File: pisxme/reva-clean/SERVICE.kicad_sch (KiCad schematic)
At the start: 5 parts, among them J4 10171746-00021LF, U8 USB2 connector-boundary ESD, X8 SERVICE_Contract

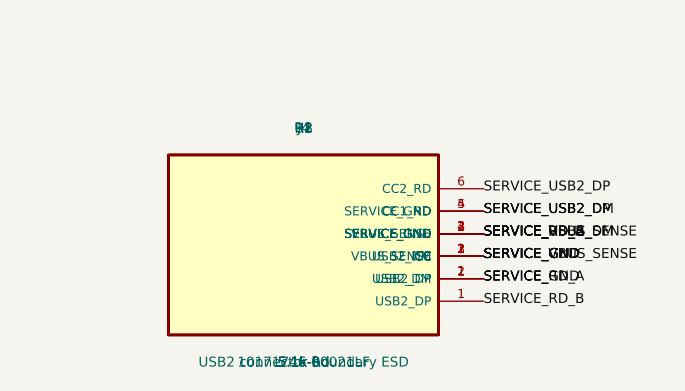
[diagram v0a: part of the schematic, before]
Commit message: close service ESD electrical authority
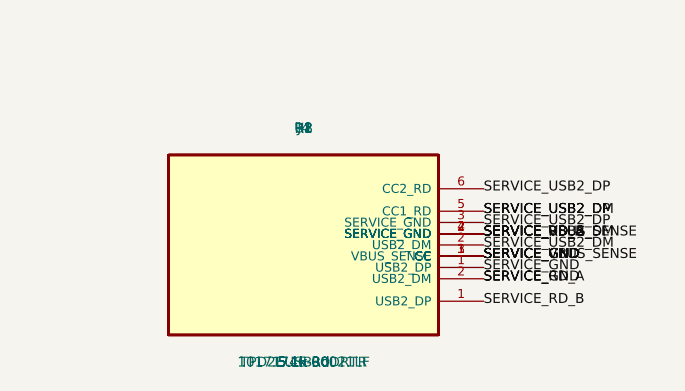
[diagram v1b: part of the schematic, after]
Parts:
- U8: value USB2 connector-boundary ESD -> TPD2EUSB30DRTR; footprint (none) -> PiSXMeRevAClean:USB_C_SERVICE_10171746; MPN USB2 connector-boundary ESD -> TPD2EUSB30DRTR
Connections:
- net SERVICE_GND: no longer U8.4 (SERVICE_GND)
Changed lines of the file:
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@@
 (label "SERVICE_VBUS_SENSE" (at 70 96.25 0) (effects (font (size 1.1 1.1)) (justify left)))
 (label "SERVICE_GND" (at 70 98.75 0) (effects (font (size 1.1 1.1)) (justify left)))
-(symbol (lib_id "PiSXMeRevAClean:USB2_ESD") (at 50 95 0) (unit 1) (exclude_from_sim no) (in_bom yes) (on_board yes) (dnp no) (property "Reference" "U8" (at 50 82 0) (effects (font (size 1.1 1.1)))) (property "Value" "USB2 connector-boundary ESD" (at 50 108 0) (effects (font (size 1.1 1.1)))) (property "MPN" "USB2 connector-boundary ESD" (at 50 95 0) (effects (font (size 1 1)) (hide yes))) (property "Footprint" "" (at 50 95 0) (effects (font (size 1 1)) (hide yes))) (pin "1")
+(label "SERVICE_USB2_DP" (at 70 92.5 0) (effects (font (size 1.1 1.1)) (justify left)))
+(label "SERVICE_USB2_DM" (at 70 95 0) (effects (font (size 1.1 1.1)) (justify left)))
+(label "SERVICE_GND" (at 70 97.5 0) (effects (font (size 1.1 1.1)) (justify left)))
+(symbol (lib_id "PiSXMeRevAClean:USB2_ESD") (at 50 95 0) (unit 1) (exclude_from_sim no) (in_bom yes) (on_board yes) (dnp no) (property "Reference" "U8" (at 50 82 0) (effects (font (size 1.1 1.1)))) (property "Value" "TPD2EUSB30DRTR" (at 50 108 0) (effects (font (size 1.1 1.1)))) (property "MPN" "TPD2EUSB30DRTR" (at 50 95 0) (effects (font (size 1 1)) (hide yes))) (property "Footprint" "PiSXMeRevAClean:USB_C_SERVICE_10171746" (at 50 95 0) (effects (font (size 1 1)) (hide yes))) (pin "1")
 (pin "2")
-(pin "3")
-(pin "4") (instances (project "PiSXMe_RevA_Clean" (path "/30000000-0000-0000-0000-000000000000" (reference "U8") (unit 1)))) )(label "SERVICE_RD_A" (at 70 93.75 0) (effects (font (size 1.1 1.1)) (justify left)))
+(pin "3") (instances (project "PiSXMe_RevA_Clean" (path "/30000000-0000-0000-0000-000000000000" (reference "U8") (unit 1)))) )(label "SERVICE_RD_A" (at 70 93.75 0) (effects (font (size 1.1 1.1)) (justify left)))
 (label "SERVICE_GND" (at 70 96.25 0) (effects (font (size 1.1 1.1)) (justify left)))
 (symbol (lib_id "PiSXMeRevAClean:USB2_RD_5K1") (at 50 95 0) (unit 1) (exclude_from_sim no) (in_bom yes) (on_board yes) (dnp no) (property "Reference" "R1" (at 50 82 0) (effects (font (size 1.1 1.1)))) (property "Value" "5.1k Rd" (at 50 108 0) (effects (font (size 1.1 1.1)))) (property "MPN" "5.1k Rd" (at 50 95 0) (effects (font (size 1 1)) (hide yes))) (property "Footprint" "PiSXMeRevAClean:USB_C_SERVICE_10171746" (at 50 95 0) (effects (font (size 1 1)) (hide yes))) (pin "1")

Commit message: close service ESD footprint authority
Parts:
- R1: footprint PiSXMeRevAClean:USB_C_SERVICE_10171746 -> PiSXMeRevAClean:R_0402_1005Metric
- R2: footprint (none) -> PiSXMeRevAClean:R_0402_1005Metric
- U8: footprint PiSXMeRevAClean:USB_C_SERVICE_10171746 -> PiSXMeRevAClean:Texas_DRT_3
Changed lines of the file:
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@@
 (label "SERVICE_USB2_DM" (at 70 95 0) (effects (font (size 1.1 1.1)) (justify left)))
 (label "SERVICE_GND" (at 70 97.5 0) (effects (font (size 1.1 1.1)) (justify left)))
-(symbol (lib_id "PiSXMeRevAClean:USB2_ESD") (at 50 95 0) (unit 1) (exclude_from_sim no) (in_bom yes) (on_board yes) (dnp no) (property "Reference" "U8" (at 50 82 0) (effects (font (size 1.1 1.1)))) (property "Value" "TPD2EUSB30DRTR" (at 50 108 0) (effects (font (size 1.1 1.1)))) (property "MPN" "TPD2EUSB30DRTR" (at 50 95 0) (effects (font (size 1 1)) (hide yes))) (property "Footprint" "PiSXMeRevAClean:USB_C_SERVICE_10171746" (at 50 95 0) (effects (font (size 1 1)) (hide yes))) (pin "1")
+(symbol (lib_id "PiSXMeRevAClean:USB2_ESD") (at 50 95 0) (unit 1) (exclude_from_sim no) (in_bom yes) (on_board yes) (dnp no) (property "Reference" "U8" (at 50 82 0) (effects (font (size 1.1 1.1)))) (property "Value" "TPD2EUSB30DRTR" (at 50 108 0) (effects (font (size 1.1 1.1)))) (property "MPN" "TPD2EUSB30DRTR" (at 50 95 0) (effects (font (size 1 1)) (hide yes))) (property "Footprint" "PiSXMeRevAClean:Texas_DRT_3" (at 50 95 0) (effects (font (size 1 1)) (hide yes))) (pin "1")
 (pin "2")
 (pin "3") (instances (project "PiSXMe_RevA_Clean" (path "/30000000-0000-0000-0000-000000000000" (reference "U8") (unit 1)))) )(label "SERVICE_RD_A" (at 70 93.75 0) (effects (font (size 1.1 1.1)) (justify left)))
 (label "SERVICE_GND" (at 70 96.25 0) (effects (font (size 1.1 1.1)) (justify left)))
-(symbol (lib_id "PiSXMeRevAClean:USB2_RD_5K1") (at 50 95 0) (unit 1) (exclude_from_sim no) (in_bom yes) (on_board yes) (dnp no) (property "Reference" "R1" (at 50 82 0) (effects (font (size 1.1 1.1)))) (property "Value" "5.1k Rd" (at 50 108 0) (effects (font (size 1.1 1.1)))) (property "MPN" "5.1k Rd" (at 50 95 0) (effects (font (size 1 1)) (hide yes))) (property "Footprint" "PiSXMeRevAClean:USB_C_SERVICE_10171746" (at 50 95 0) (effects (font (size 1 1)) (hide yes))) (pin "1")
+(symbol (lib_id "PiSXMeRevAClean:USB2_RD_5K1") (at 50 95 0) (unit 1) (exclude_from_sim no) (in_bom yes) (on_board yes) (dnp no) (property "Reference" "R1" (at 50 82 0) (effects (font (size 1.1 1.1)))) (property "Value" "5.1k Rd" (at 50 108 0) (effects (font (size 1.1 1.1)))) (property "MPN" "5.1k Rd" (at 50 95 0) (effects (font (size 1 1)) (hide yes))) (property "Footprint" "PiSXMeRevAClean:R_0402_1005Metric" (at 50 95 0) (effects (font (size 1 1)) (hide yes))) (pin "1")
 (pin "2") (instances (project "PiSXMe_RevA_Clean" (path "/30000000-0000-0000-0000-000000000000" (reference "R1") (unit 1)))) )(label "SERVICE_RD_B" (at 70 93.75 0) (effects (font (size 1.1 1.1)) (justify left)))
 (label "SERVICE_GND" (at 70 96.25 0) (effects (font (size 1.1 1.1)) (justify left)))
-(symbol (lib_id "PiSXMeRevAClean:USB2_RD_5K1") (at 50 95 0) (unit 1) (exclude_from_sim no) (in_bom yes) (on_board yes) (dnp no) (property "Reference" "R2" (at 50 82 0) (effects (font (size 1.1 1.1)))) (property "Value" "5.1k Rd" (at 50 108 0) (effects (font (size 1.1 1.1)))) (property "MPN" "5.1k Rd" (at 50 95 0) (effects (font (size 1 1)) (hide yes))) (property "Footprint" "" (at 50 95 0) (effects (font (size 1 1)) (hide yes))) (pin "1")
+(symbol (lib_id "PiSXMeRevAClean:USB2_RD_5K1") (at 50 95 0) (unit 1) (exclude_from_sim no) (in_bom yes) (on_board yes) (dnp no) (property "Reference" "R2" (at 50 82 0) (effects (font (size 1.1 1.1)))) (property "Value" "5.1k Rd" (at 50 108 0) (effects (font (size 1.1 1.1)))) (property "MPN" "5.1k Rd" (at 50 95 0) (effects (font (size 1 1)) (hide yes))) (property "Footprint" "PiSXMeRevAClean:R_0402_1005Metric" (at 50 95 0) (effects (font (size 1 1)) (hide yes))) (pin "1")
 (pin "2") (instances (project "PiSXMe_RevA_Clean" (path "/30000000-0000-0000-0000-000000000000" (reference "R2") (unit 1)))) )
   (sheet_instances (path "/30000000-0000-0000-0000-000000000000/10000000-0000-0000-0000-000000000008" (page "8")))
